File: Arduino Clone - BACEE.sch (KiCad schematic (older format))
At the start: 13 parts, among them U1 24LC1025, U2 24LC1025, U3 DS13375+, U4 ATMEGA328P-AU, Y1 Crystal 32Mhz, Y2 Crystal 16Mhz

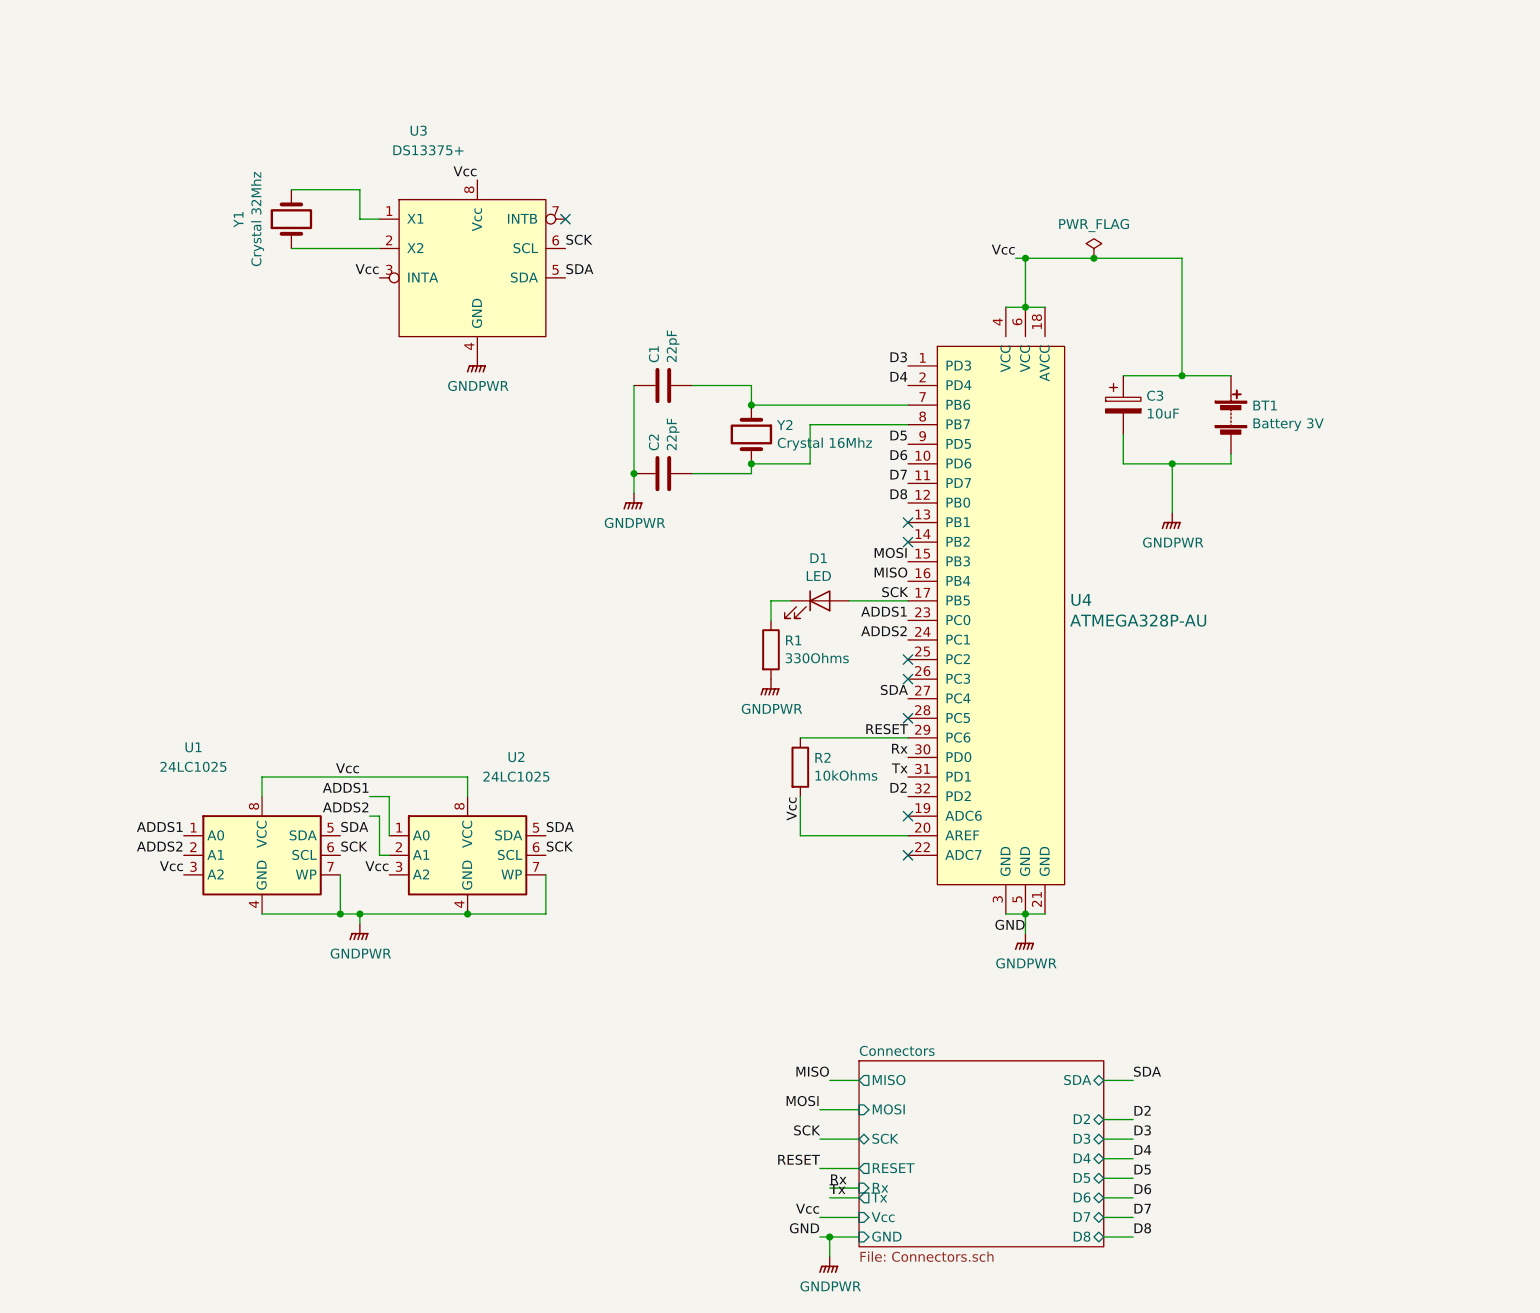
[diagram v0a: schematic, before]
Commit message: Comments
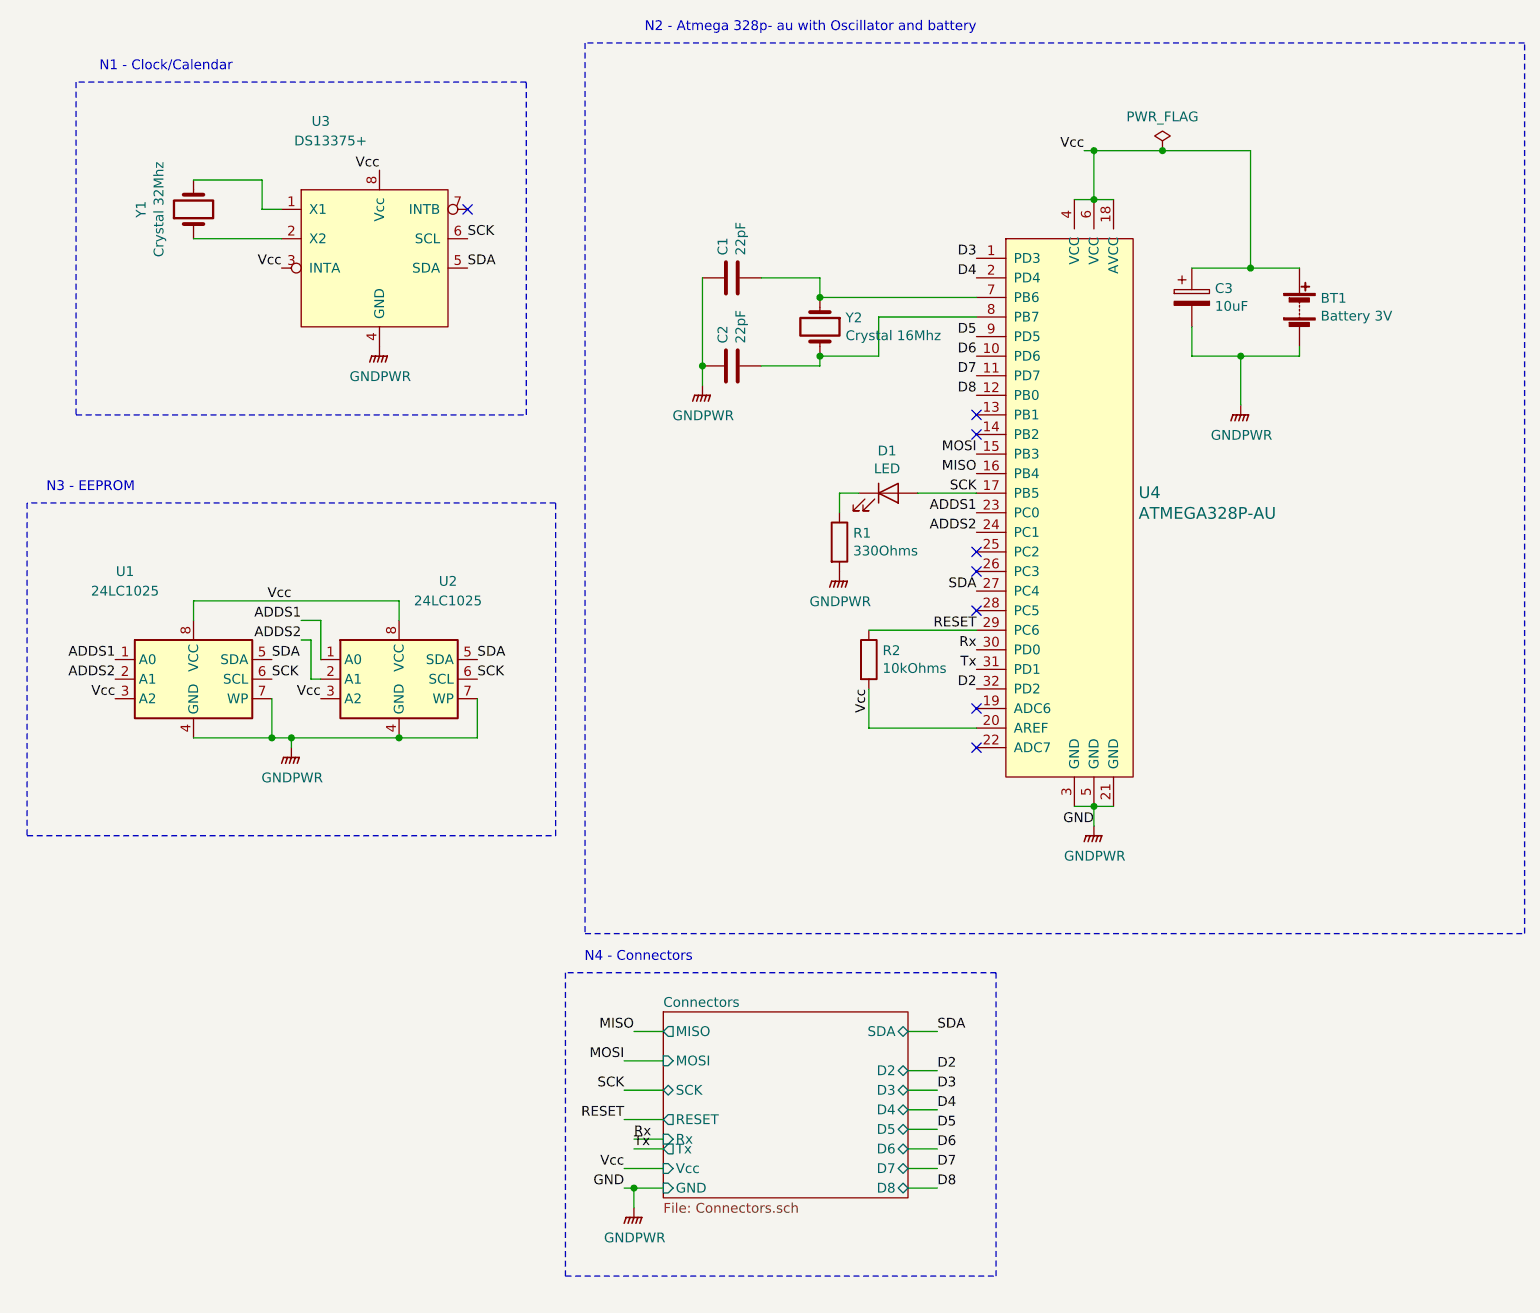
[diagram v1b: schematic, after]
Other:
- note added: "N1 - Clock/Calendar\n"
- note added: "N2 - Atmega 328p- au with Oscillator and battery"
- note added: "N3 - EEPROM\n"
- note added: "N4 - Connectors"
- moved on the sheet: BT1, C1, C2, C3, D1, R1, R2, U1, U2, U3, U4, Y1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
